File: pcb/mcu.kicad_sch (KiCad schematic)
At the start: 33 parts, among them J1 Conn_01x02_Pin, SW1 SW_SPDT, SW2 SW_Push, SW3 SW_SPDT, U1 TLV1117LV33DCYR, U2 W25Q64JVSSIQ_C179171, U3 STM32H750VBTx, Y1 25 MHz

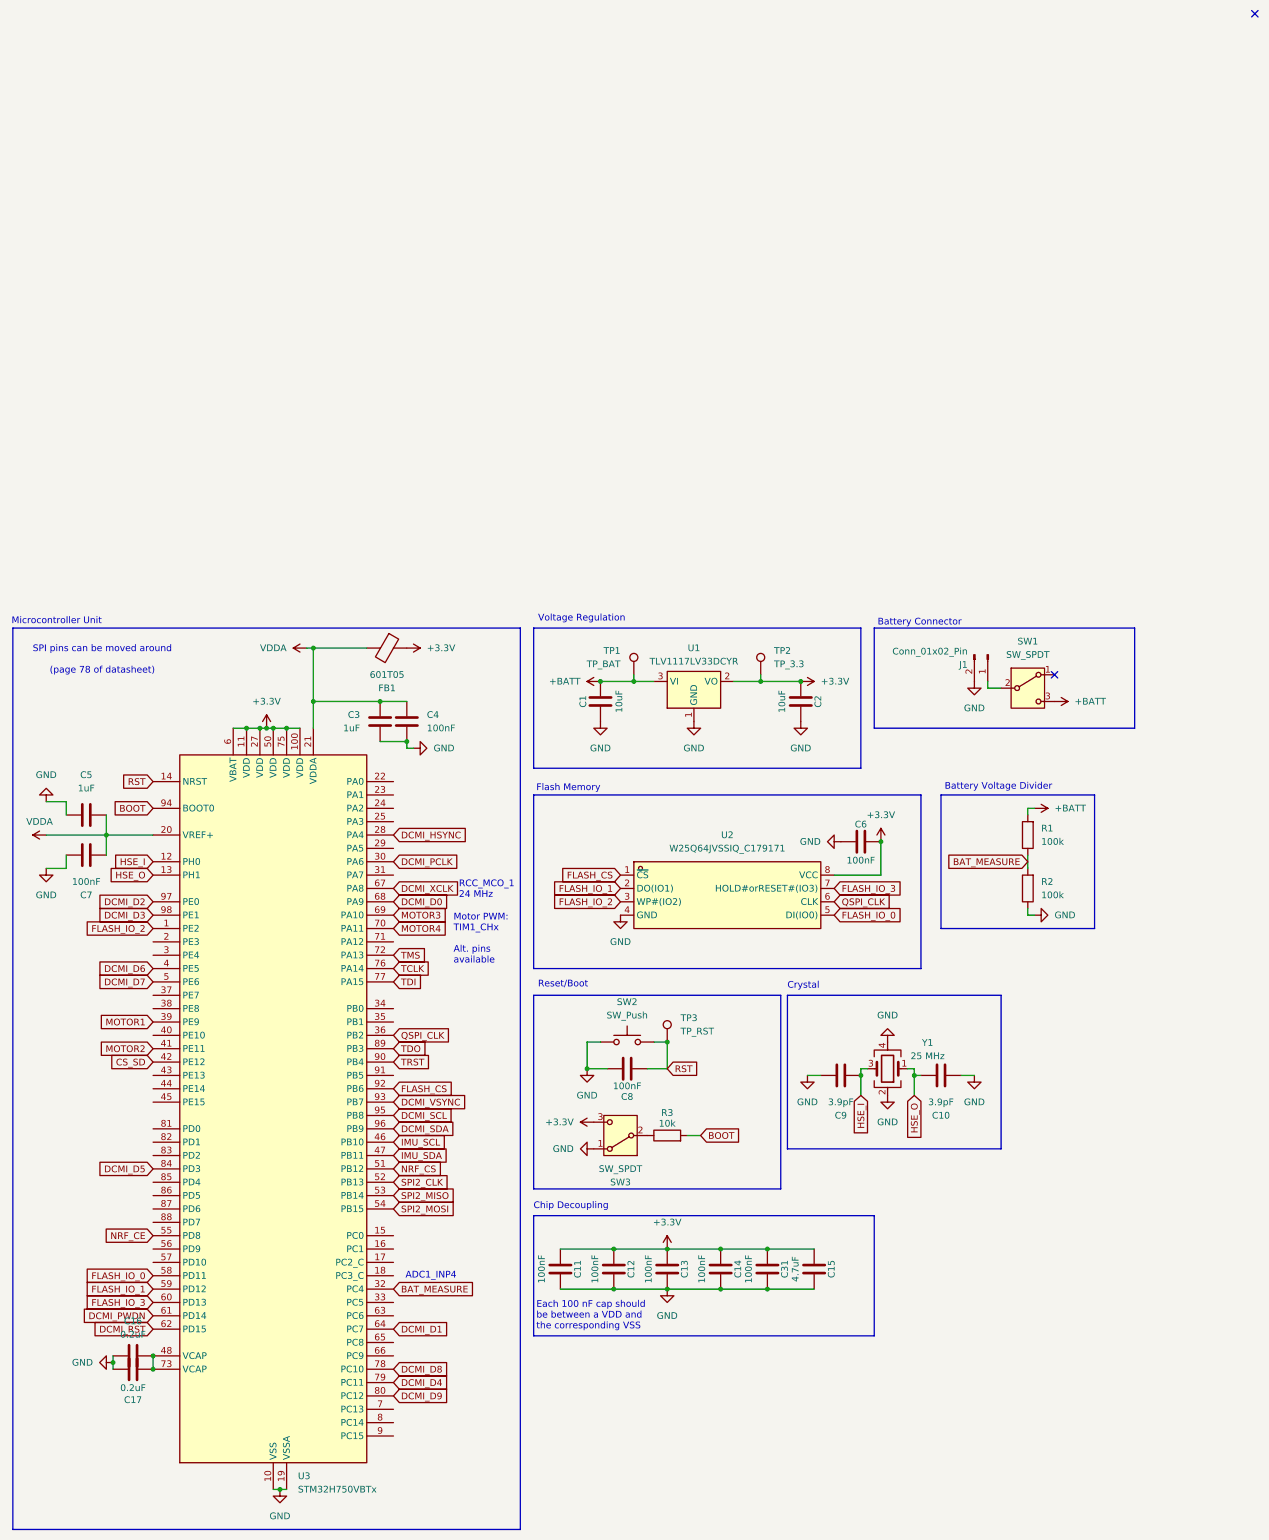
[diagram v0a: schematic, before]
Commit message: [pcb] invented the cutting edge, extremely innovative monke and ddg connectors
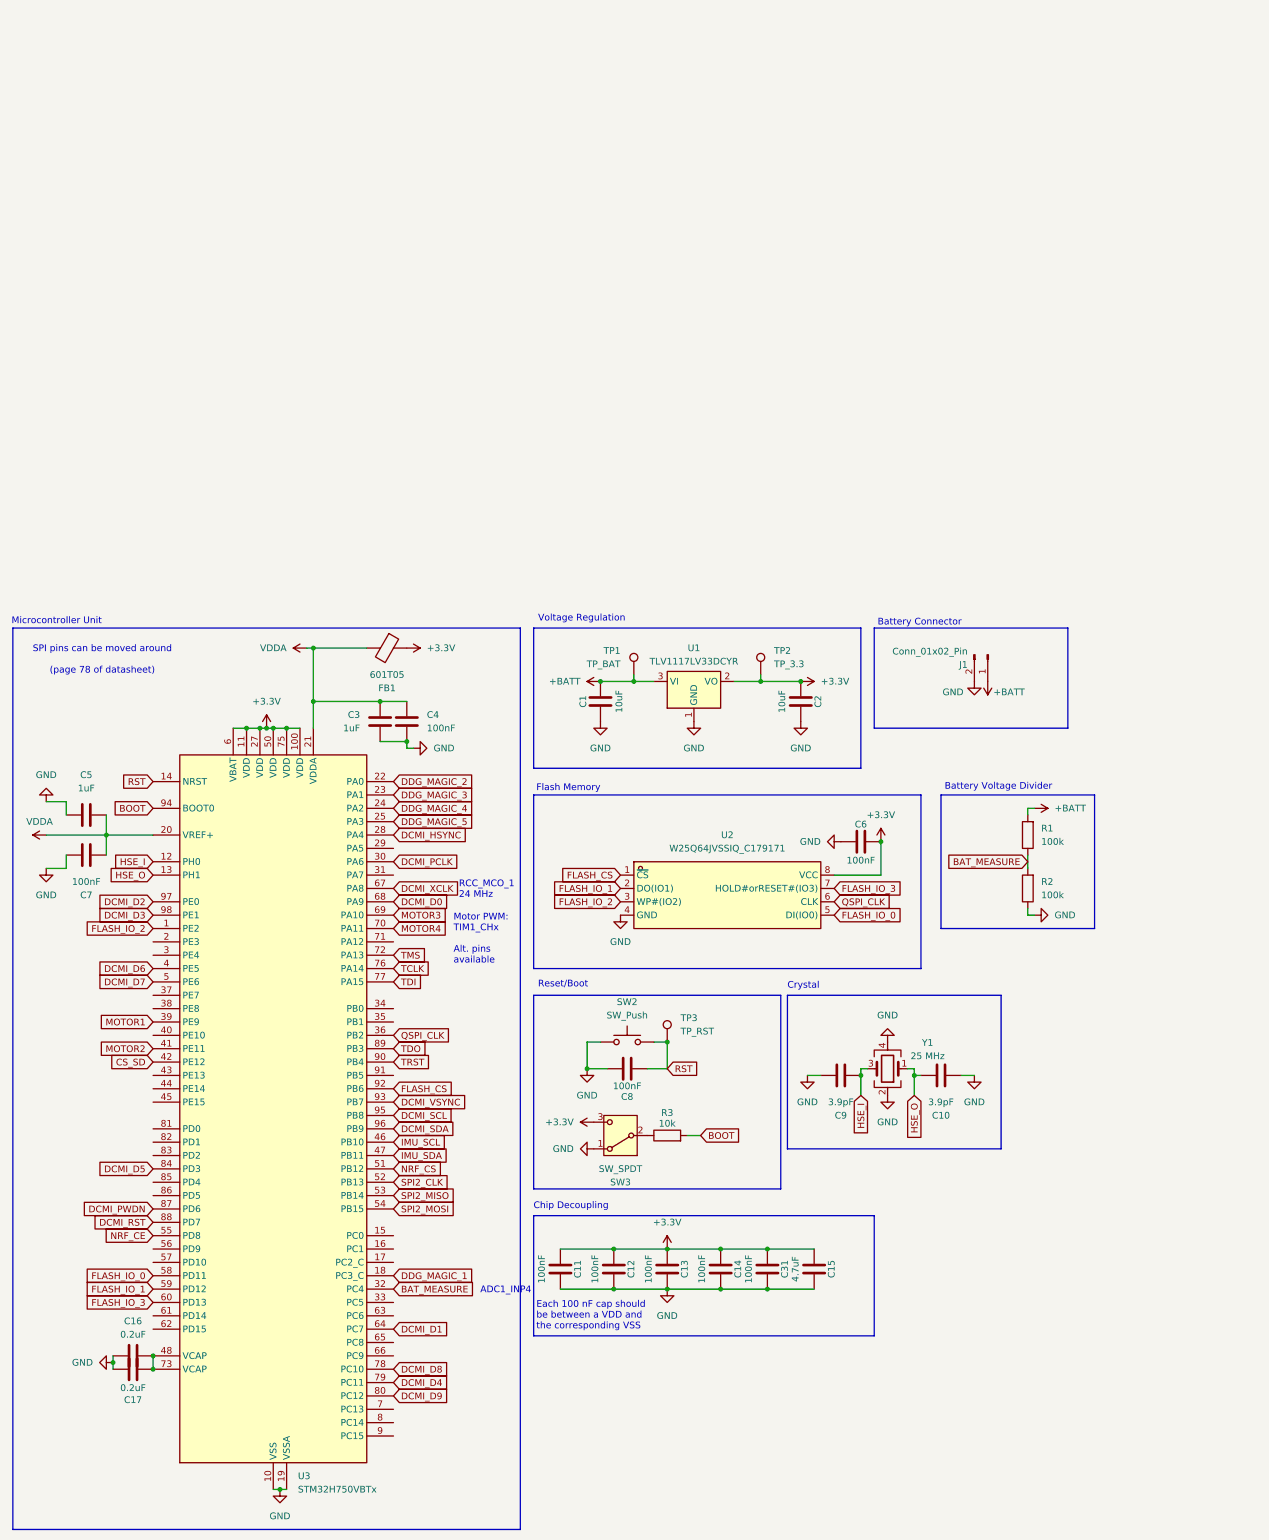
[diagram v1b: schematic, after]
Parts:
- removed SW1: SW_SPDT, Button_Switch_THT:SW_Slide-03_Wuerth-WS-SLTV_10x2.5x6.4_P2.54mm, symbol Switch:SW_SPDT
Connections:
- net +BATT: now also J1.1 (Pin_1)
- net DCMI_PWDN: now also U3.87 (PD6); no longer U3.61 (PD14)
- net DCMI_RST: now also U3.88 (PD7); no longer U3.62 (PD15)
- net DDG_MAGIC_1: now reaches U3.18 (PC3_C)
- net DDG_MAGIC_2: now reaches U3.22 (PA0)
- net DDG_MAGIC_3: now reaches U3.23 (PA1)
- net DDG_MAGIC_4: now reaches U3.24 (PA2)
- net DDG_MAGIC_5: now reaches U3.25 (PA3)
- no-connect marks 2 -> 0
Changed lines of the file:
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@@
 	(rectangle
 		(start 179.07 16.51)
-		(end 228.6 35.56)
+		(end 215.9 35.56)
 		(stroke
 			(width 0)
@@
 	(text "ADC1_INP4"
 		(exclude_from_sim no)
-		(at 89.916 139.7 0)
+		(at 104.14 142.494 0)
 		(effects
 			(font
@@
 		(color 0 0 0 0)
 	)
-	(no_connect
-		(at 251.46 -100.33)
-	)
-	(no_connect
-		(at 213.36 25.4)
-	)
 	(wire
 		(pts
@@
 	(wire
 		(pts
-			(xy 200.66 26.67) (xy 200.66 27.94)
-		)
-		(stroke
-			(width 0)
-			(type default)
-		)
-	)
-	(wire
-		(pts
 			(xy 124.46 100.33) (xy 124.46 95.25)
 		)
@@
 	(wire
 		(pts
-			(xy 200.66 27.94) (xy 203.2 27.94)
-		)
-		(stroke
-			(width 0)
-			(type default)
-		)
-	)
-	(wire
-		(pts
 			(xy 66.04 180.34) (xy 64.77 180.34)
 		)
@@
 		)
 	)
+	(global_label "DDG_MAGIC_4"
+		(shape input)
+		(at 87.63 50.8 0)
+		(fields_autoplaced yes)
+		(effects
+			(font
+				(size 1.27 1.27)
+			)
+			(justify left)
+		)
+		(property "Intersheetrefs" "${INTERSHEET_REFS}"
+			(at 103.2547 50.8 0)
+			(effects
+				(font
+					(size 1.27 1.27)
+				)
+				(justify left)
+				(hide yes)
+			)
+		)
+	)
 	(global_label "FLASH_IO_1"
 		(shape input)
@@
 		)
 	)
+	(global_label "DCMI_RST"
+		(shape input)
+		(at 41.91 129.54 180)
+		(fields_autoplaced yes)
+		(effects
+			(font
+				(size 1.27 1.27)
+			)
+			(justify right)
+		)
+		(property "Intersheetrefs" "${INTERSHEET_REFS}"
+			(at 29.9139 129.54 0)
+			(effects
+				(font
+					(size 1.27 1.27)
+				)
+				(justify right)
+				(hide yes)
+			)
+		)
+	)
 	(global_label "TMS"
 		(shape input)
@@
 		)
 	)
+	(global_label "DCMI_PWDN"
+		(shape input)
+		(at 41.91 127 180)
+		(fields_autoplaced yes)
+		(effects
+			(font
+				(size 1.27 1.27)
+			)
+			(justify right)
+		)
+		(property "Intersheetrefs" "${INTERSHEET_REFS}"
+			(at 28.0391 127 0)
+			(effects
+				(font
+					(size 1.27 1.27)
+				)
+				(justify right)
+				(hide yes)
+			)
+		)
+	)
 	(global_label "MOTOR4"
 		(shape input)
@@
 		)
 	)
+	(global_label "DDG_MAGIC_2"
+		(shape input)
+		(at 87.63 45.72 0)
+		(fields_autoplaced yes)
+		(effects
+			(font
+				(size 1.27 1.27)
+			)
+			(justify left)
+		)
+		(property "Intersheetrefs" "${INTERSHEET_REFS}"
+			(at 103.2547 45.72 0)
+			(effects
+				(font
+					(size 1.27 1.27)
+				)
+				(justify left)
+				(hide yes)
+			)
+		)
+	)
 	(global_label "DCMI_PCLK"
 		(shape input)
@@
 		)
 	)
-	(global_label "DCMI_RST"
+	(global_label "DDG_MAGIC_1"
 		(shape input)
-		(at 41.91 149.86 180)
+		(at 87.63 139.7 0)
 		(fields_autoplaced yes)
 		(effects
@@
 				(size 1.27 1.27)
 			)
-			(justify right)
+			(justify left)
 		)
 		(property "Intersheetrefs" "${INTERSHEET_REFS}"
-			(at 29.9139 149.86 0)
+			(at 103.2547 139.7 0)
 			(effects
 				(font
 					(size 1.27 1.27)
 				)
-				(justify right)
+				(justify left)
 				(hide yes)
 			)
@@
 		)
 	)
+	(global_label "DDG_MAGIC_5"
+		(shape input)
+		(at 87.63 53.34 0)
+		(fields_autoplaced yes)
+		(effects
+			(font
+				(size 1.27 1.27)
+			)
+			(justify left)
+		)
+		(property "Intersheetrefs" "${INTERSHEET_REFS}"
+			(at 103.2547 53.34 0)
+			(effects
+				(font
+					(size 1.27 1.27)
+				)
+				(justify left)
+				(hide yes)
+			)
+		)
+	)
 	(global_label "MOTOR3"
 		(shape input)
@@
 		)
 	)
-	(global_label "HSE_I"
+	(global_label "DDG_MAGIC_3"
 		(shape input)
-		(at 41.91 60.96 180)
+		(at 87.63 48.26 0)
 		(fields_autoplaced yes)
 		(effects
@@
 				(size 1.27 1.27)
 			)
-			(justify right)
+			(justify left)
 		)
 		(property "Intersheetrefs" "${INTERSHEET_REFS}"
-			(at 33.6634 60.96 0)
+			(at 103.2547 48.26 0)
 			(effects
 				(font
 					(size 1.27 1.27)
 				)
-				(justify right)
+				(justify left)
 				(hide yes)
 			)
 		)
 	)
-	(global_label "DCMI_HSYNC"
+	(global_label "HSE_I"
 		(shape input)
-		(at 87.63 55.88 0)
+		(at 41.91 60.96 180)
 		(fields_autoplaced yes)
 		(effects
@@
 				(size 1.27 1.27)
 			)
-			(justify left)
+			(justify right)
 		)
 		(property "Intersheetrefs" "${INTERSHEET_REFS}"
-			(at 102.4081 55.88 0)
+			(at 33.6634 60.96 0)
 			(effects
 				(font
 					(size 1.27 1.27)
 				)
-				(justify left)
+				(justify right)
 				(hide yes)
 			)
 		)
 	)
-	(global_label "DCMI_PWDN"
+	(global_label "DCMI_HSYNC"
 		(shape input)
-		(at 41.91 147.32 180)
+		(at 87.63 55.88 0)
 		(fields_autoplaced yes)
 		(effects
@@
 				(size 1.27 1.27)
 			)
-			(justify right)
+			(justify left)
 		)
 		(property "Intersheetrefs" "${INTERSHEET_REFS}"
-			(at 28.0391 147.32 0)
+			(at 102.4081 55.88 0)
 			(effects
 				(font
 					(size 1.27 1.27)
 				)
-				(justify right)
+				(justify left)
 				(hide yes)
 			)
@@
 	(symbol
 		(lib_id "power:+BATT")
-		(at 213.36 30.48 270)
+		(at 200.66 26.67 180)
 		(unit 1)
 		(exclude_from_sim no)
@@
 		(on_board yes)
 		(dnp no)
-		(fields_autoplaced yes)
 		(property "Reference" "#PWR06"
-			(at 209.55 30.48 0)
+			(at 200.66 22.86 0)
 			(effects
 				(font
@@
 		)
 		(property "Value" "+BATT"
-			(at 217.17 30.4799 90)
+			(at 204.724 28.702 0)
 			(effects
 				(font
 					(size 1.27 1.27)
 				)
-				(justify left)
 			)
 		)
 		(property "Footprint" ""
-			(at 213.36 30.48 0)
+			(at 200.66 26.67 0)
 			(effects
 				(font
@@
 		)
 		(property "Datasheet" ""
-			(at 213.36 30.48 0)
+			(at 200.66 26.67 0)
 			(effects
 				(font
@@
 		)
 		(property "Description" "Power symbol creates a global label with name \"+BATT\""
-			(at 213.36 30.48 0)
+			(at 200.66 26.67 0)
 			(effects
 				(font
@@
 		(on_board yes)
 		(dnp no)
-		(fields_autoplaced yes)
 		(property "Reference" "#PWR05"
 			(at 198.12 33.02 0)
@@
 		)
 		(property "Value" "GND"
-			(at 198.12 31.75 0)
+			(at 194.056 28.702 0)
 			(effects
 				(font
@@
 					(unit 1)
 				)
-			)
-		)
-	)
-	(symbol
-		(lib_id "Switch:SW_SPDT")
-		(at 208.28 27.94 0)
-		(unit 1)
-		(exclude_from_sim no)
-		(in_bom yes)
-		(on_board yes)
-		(dnp no)
-		(fields_autoplaced yes)
-		(property "Reference" "SW1"
-			(at 208.28 19.05 0)
-			(effects
-				(font
-					(size 1.27 1.27)
-				)
-			)
-		)
-		(property "Value" "SW_SPDT"
-			(at 208.28 21.59 0)
-			(effects
-				(font
-					(size 1.27 1.27)
-				)
-			)
-		)
-		(property "Footprint" "Button_Switch_THT:SW_Slide-03_Wuerth-WS-SLTV_10x2.5x6.4_P2.54mm"
-			(at 208.28 27.94 0)
-			(effects
-				(font
-					(size 1.27 1.27)
-				)
-				(hide yes)
-			)
-		)
-		(property "Datasheet" "~"
-			(at 208.28 35.56 0)
-			(effects
-				(font
-					(size 1.27 1.27)
-				)
-				(hide yes)
-			)
-		)
-		(property "Description" "Switch, single pole double throw"
-			(at 208.28 27.94 0)
-			(effects
-				(font
-					(size 1.27 1.27)
-				)
-				(hide yes)
-			)
-		)
-		(pin "2"
-		)
-		(pin "3"
-		)
-		(pin "1"
-		)
-		(instances
-			(project ""
-				(path "/c0be3de2-9de4-4447-aa6f-537ea5f31aac/0c8c942c-f992-4664-b7a3-b87cb51e1584"
-					(reference "SW1")
-					(unit 1)
-				)
